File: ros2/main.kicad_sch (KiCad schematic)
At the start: 17 parts, among them J1 Battery, U1 ESP32-DEVKIT-V1, U2 TB6612NFG, U3 TB6612NFG, U4 ACS712, U5 XL63070, U6 TXS0108E, U7 TB6612NFG, U8 TB6612NFG

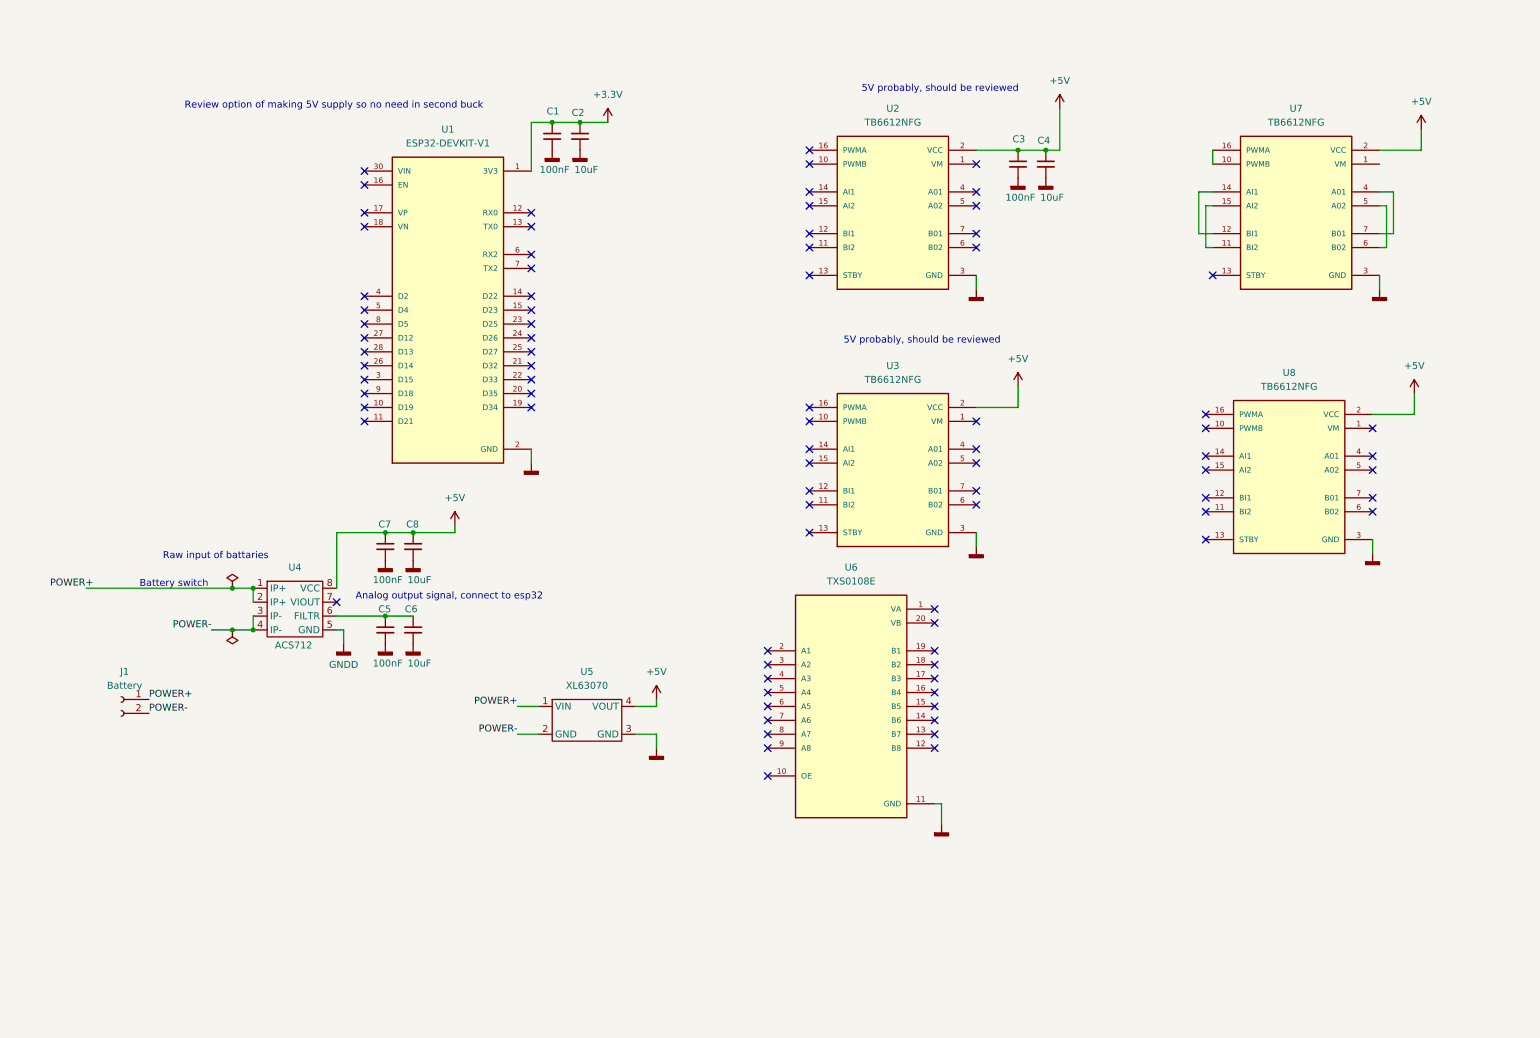
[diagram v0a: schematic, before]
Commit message: schema without esp32
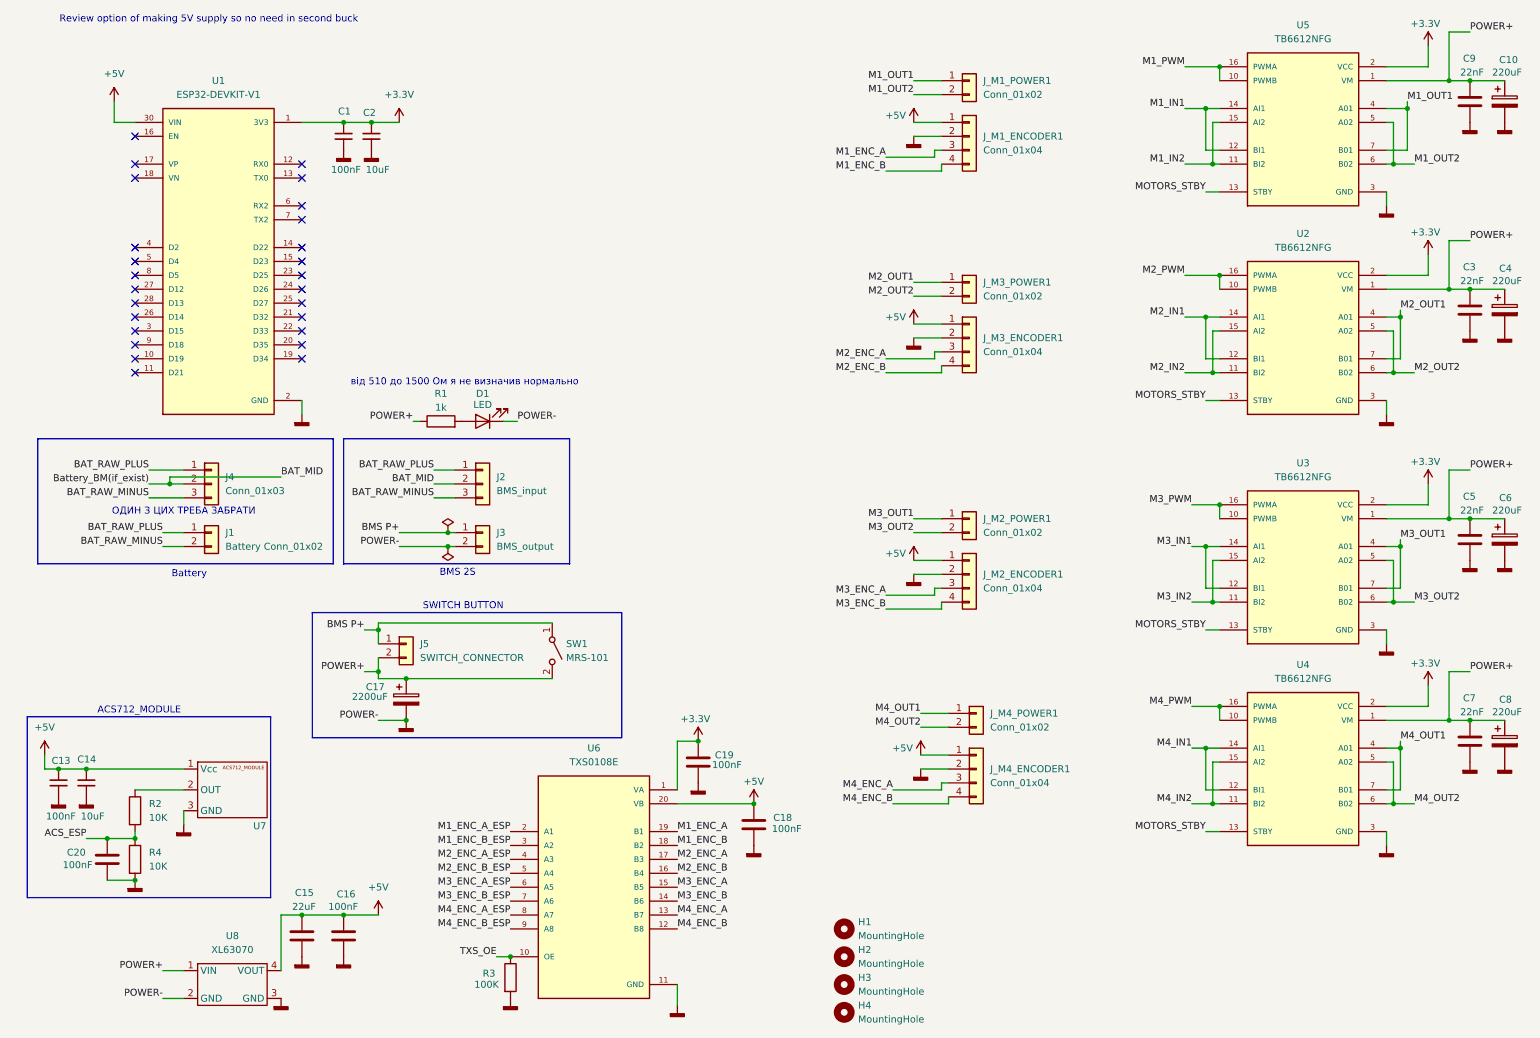
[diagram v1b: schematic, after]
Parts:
- removed C3, C5, C7: 100nF, symbol Device:C_Small
- removed C4, C6, C8: 10uF, symbol Device:C_Small
- removed J1: Battery, Battery:Connector, symbol Connector:Conn_01x02_Socket
- removed U4: ACS712, Package_SO:SOIC-8_3.9x4.9mm_P1.27mm, symbol ACS712:ACS712
- removed U8: TB6612NFG, tb6612fng:MODULE_ROB-14450, symbol ROB-14450:ROB-14450
- added C10, C4, C6, C8: 220uF, symbol Device:C_Polarized
- added C13: 100nF, symbol Device:C_Small
- added C14: 10uF, symbol Device:C_Small
- added C15: 22uF, symbol Device:C
- added C16, C18, C19, C20: 100nF, symbol Device:C
- added C17: 2200uF, symbol Device:C_Polarized
- added C3, C5, C7, C9: 22nF, symbol Device:C
- added D1: LED, symbol Device:LED
- added H1, H2, H3, H4: MountingHole, symbol Mechanical:MountingHole
- added J1: Battery Conn_01x02, TerminalBlock:TerminalBlock_Xinya_XY308-2.54-2P_1x02_P2.54mm_Horizontal, symbol Connector_Generic:Conn_01x02
- added J2: BMS_input, Connector_Wire:SolderWire-1sqmm_1x03_P5.4mm_D1.4mm_OD2.7mm, symbol Connector_Generic:Conn_01x03
- added J3: BMS_output, Connector_Wire:SolderWire-1sqmm_1x02_P5.4mm_D1.4mm_OD2.7mm, symbol Connector_Generic:Conn_01x02
- added J4: Conn_01x03, symbol Connector_Generic:Conn_01x03
- added J5: SWITCH_CONNECTOR, Connector_Wire:SolderWire-1sqmm_1x02_P5.4mm_D1.4mm_OD2.7mm, symbol Connector_Generic:Conn_01x02
- added J_M1_ENCODER1, J_M2_ENCODER1, J_M3_ENCODER1, J_M4_ENCODER1: Conn_01x04, Connector_PinHeader_2.54mm:PinHeader_1x04_P2.54mm_Vertical, symbol Connector_Generic:Conn_01x04
- added J_M1_POWER1, J_M2_POWER1, J_M3_POWER1, J_M4_POWER1: Conn_01x02, TerminalBlock:TerminalBlock_Xinya_XY308-2.54-2P_1x02_P2.54mm_Horizontal, symbol Connector_Generic:Conn_01x02
- added R1: 1k, symbol Device:R
- added R2, R4: 10K, symbol Device:R
- added R3: 100K, symbol Device:R
- added SW1: MRS-101, symbol Switch:SW_SPST
- added U5: TB6612NFG, tb6612fng:MODULE_ROB-14450, symbol ROB-14450:ROB-14450
- added U7: (no value), ACS712_MODULE:ACS712_module, symbol ACS712_Module:ACS712_30A
- renumbered U7 to U4, U5 to U8
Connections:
- net POWER- is gone; now on net GND: U8.2 (GND)
- net +3.3V: now also U2.2 (VCC), U3.2 (VCC), U4.2 (VCC), U6.1 (VA), C19.1, U5.2 (VCC)
- net +5V: now also U1.30 (VIN), U6.20 (VB), C13.1, C14.1, C15.1, C16.1, C18.1, J_M1_ENCODER1.1 (Pin_1), J_M2_ENCODER1.1 (Pin_1), J_M3_ENCODER1.1 (Pin_1), J_M4_ENCODER1.1 (Pin_1), U7.1 (Vcc); no longer U2.2 (VCC), U3.2 (VCC), U4.2 (VCC)
- net GND: now also C10.2, C13.2, C14.2, C15.2, C16.2, C17.2, C18.2, C19.2, C20.2, C3.2, C4.2, C5.2, C6.2, C7.2, C8.2, C9.2, D1.1 (K), J3.2 (Pin_2), J_M1_ENCODER1.2 (Pin_2), J_M2_ENCODER1.2 (Pin_2), J_M3_ENCODER1.2 (Pin_2), J_M4_ENCODER1.2 (Pin_2), R3.2, R4.2, U5.3 (GND), U5.8 (GND), U5.9 (GND), U7.3 (GND)
- net POWER+: now also U2.1 (VM), U3.1 (VM), U4.1 (VM), C10.1, C17.1, C3.1, C4.1, C5.1, C6.1, C7.1, C8.1, C9.1, J5.2 (Pin_2), R1.1, SW1.2 (B), U5.1 (VM)
- net M4_PWM: now reaches U4.10 (PWMB), U4.16 (PWMA)
- net M4_IN2: now reaches U4.11 (BI2), U4.15 (AI2)
- net M4_IN1: now reaches U4.12 (BI1), U4.14 (AI1)
- net MOTORS_STBY: now reaches U4.13 (STBY)
- net MOTORS_STBY: now also U2.13 (STBY), U3.13 (STBY), U5.13 (STBY)
- net M4_OUT1: now reaches U4.4 (A01), U4.7 (B01)
- net M4_OUT1: now also J_M4_POWER1.1 (Pin_1)
- net M4_OUT2: now reaches U4.5 (A02), U4.6 (B02)
- net M4_OUT2: now also J_M4_POWER1.2 (Pin_2)
- net M3_PWM: now reaches U3.10 (PWMB)
- net M3_PWM: now also U3.16 (PWMA)
- net M3_IN2: now reaches U3.11 (BI2)
- net M3_IN2: now also U3.15 (AI2)
- net M3_IN1: now reaches U3.12 (BI1)
- net M3_IN1: now also U3.14 (AI1)
- net M3_OUT1: now reaches U3.4 (A01)
- net M3_OUT1: now also U3.7 (B01), J_M2_POWER1.1 (Pin_1)
- net M3_OUT2: now reaches U3.5 (A02)
- net M3_OUT2: now also U3.6 (B02), J_M2_POWER1.2 (Pin_2)
- net M2_PWM: now reaches U2.10 (PWMB)
- net M2_PWM: now also U2.16 (PWMA)
- net M2_IN2: now reaches U2.11 (BI2)
- net M2_IN2: now also U2.15 (AI2)
- net M2_IN1: now reaches U2.12 (BI1)
- net M2_IN1: now also U2.14 (AI1)
- net M2_OUT1: now reaches U2.4 (A01)
- net M2_OUT1: now also U2.7 (B01), J_M3_POWER1.1 (Pin_1)
- net M2_OUT2: now reaches U2.5 (A02)
- net M2_OUT2: now also U2.6 (B02), J_M3_POWER1.2 (Pin_2)
- net TXS_OE: now reaches U6.10 (OE)
- net TXS_OE: now also R3.1
- net M4_ENC_B: now reaches U6.12 (B8)
- net M4_ENC_B: now also J_M4_ENCODER1.4 (Pin_4)
- net M4_ENC_A: now reaches U6.13 (B7)
- net M4_ENC_A: now also J_M4_ENCODER1.3 (Pin_3)
- net M3_ENC_B: now reaches U6.14 (B6)
- net M3_ENC_B: now also J_M2_ENCODER1.4 (Pin_4)
- net M3_ENC_A: now reaches U6.15 (B5)
- net M3_ENC_A: now also J_M2_ENCODER1.3 (Pin_3)
- net M2_ENC_B: now reaches U6.16 (B4)
- net M2_ENC_B: now also J_M3_ENCODER1.4 (Pin_4)
- net M2_ENC_A: now reaches U6.17 (B3)
- net M2_ENC_A: now also J_M3_ENCODER1.3 (Pin_3)
- net M1_ENC_B: now reaches U6.18 (B2)
- net M1_ENC_B: now also J_M1_ENCODER1.4 (Pin_4)
- net M1_ENC_A: now reaches U6.19 (B1)
- net M1_ENC_A: now also J_M1_ENCODER1.3 (Pin_3)
- net M1_ENC_A_ESP: now reaches U6.2 (A1)
- net M1_ENC_B_ESP: now reaches U6.3 (A2)
- net M2_ENC_A_ESP: now reaches U6.4 (A3)
- net M2_ENC_B_ESP: now reaches U6.5 (A4)
- net M3_ENC_A_ESP: now reaches U6.6 (A5)
- net M3_ENC_B_ESP: now reaches U6.7 (A6)
- net M4_ENC_A_ESP: now reaches U6.8 (A7)
- net M4_ENC_B_ESP: now reaches U6.9 (A8)
- new net: R2.1, U7.2 (OUT)
- new net: D1.2 (A), R1.2
- new net ACS_ESP: C20.1, R2.2, R4.1
- new net BAT_MID: J2.2 (Pin_2), J4.2 (Pin_2)
- new net BAT_RAW_MINUS: J1.2 (Pin_2), J2.3 (Pin_3), J4.3 (Pin_3)
- new net BAT_RAW_PLUS: J1.1 (Pin_1), J2.1 (Pin_1), J4.1 (Pin_1)
- new net BMS P+: J3.1 (Pin_1), J5.1 (Pin_1), SW1.1 (A)
- new net M1_IN1: U5.12 (BI1), U5.14 (AI1)
- new net M1_IN2: U5.11 (BI2), U5.15 (AI2)
- new net M1_OUT1: J_M1_POWER1.1 (Pin_1), U5.4 (A01), U5.7 (B01)
- new net M1_OUT2: J_M1_POWER1.2 (Pin_2), U5.5 (A02), U5.6 (B02)
- new net M1_PWM: U5.10 (PWMB), U5.16 (PWMA)
- no-connect marks 84 -> 26
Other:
- note added: "ACS712_MODULE"
- note added: "BMS 2S"
- note added: "Battery"
- note added: "SWITCH BUTTON"
- note added: "ОДИН З ЦИХ ТРЕБА ЗАБРАТИ"
- note added: "від 510 до 1500 Ом я не визначив нормально"
- note removed: "5V probably, should be reviewed"
- note removed: "Analog output signal, connect to esp32"
- note removed: "Battery switch"
- note removed: "Raw input of battaries"
- moved on the sheet: C1, C2, U1, U4, U6, U8
